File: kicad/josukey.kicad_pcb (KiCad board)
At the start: 2 copper layers, 150.9 x 94.8 mm, 44 parts

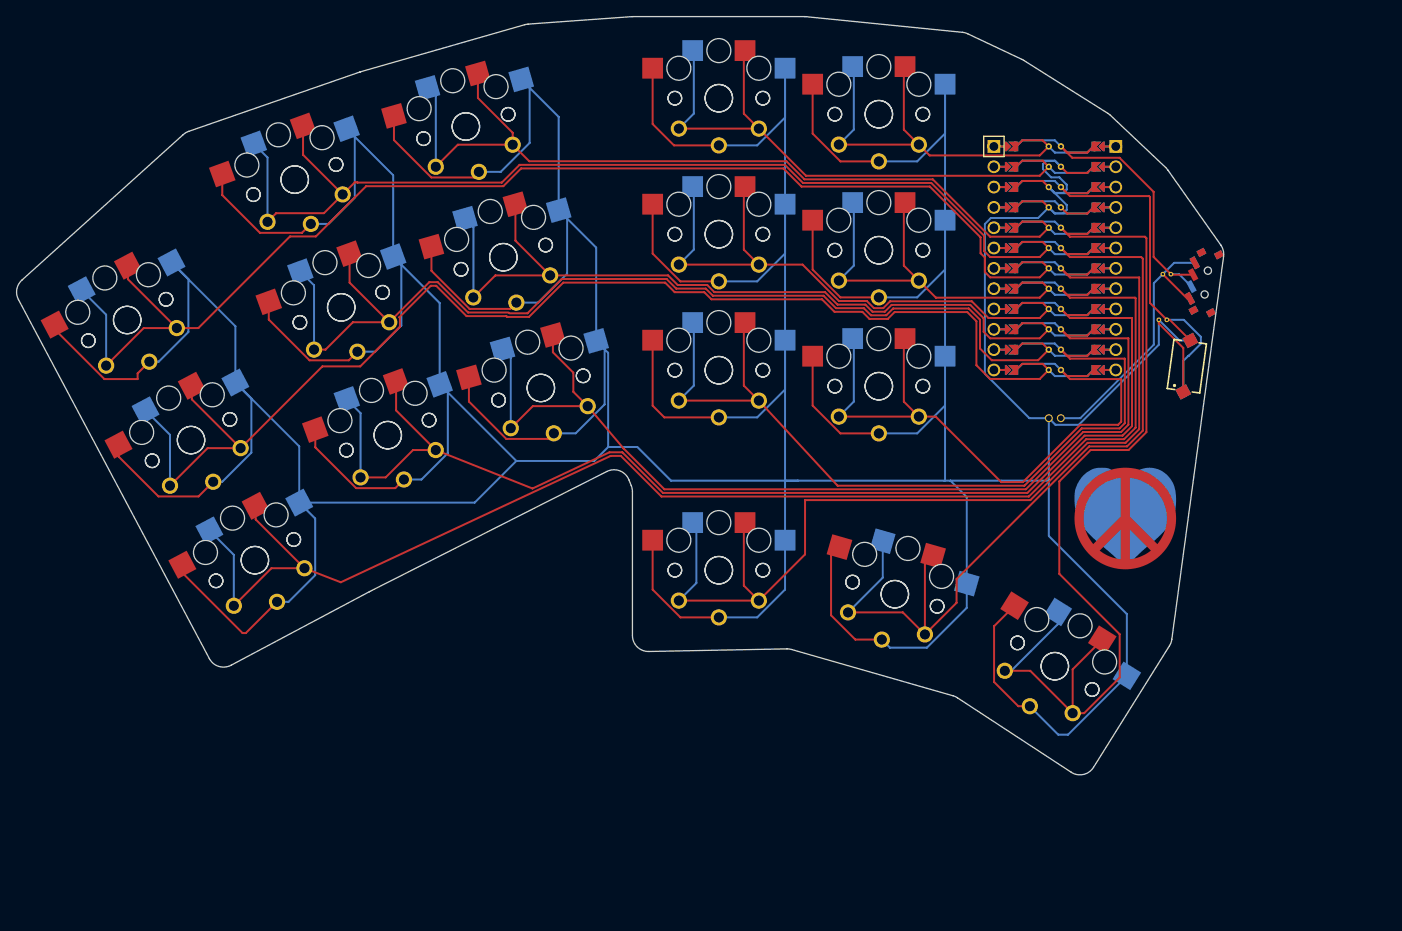
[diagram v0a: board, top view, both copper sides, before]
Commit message: add text and include images in ergogen config
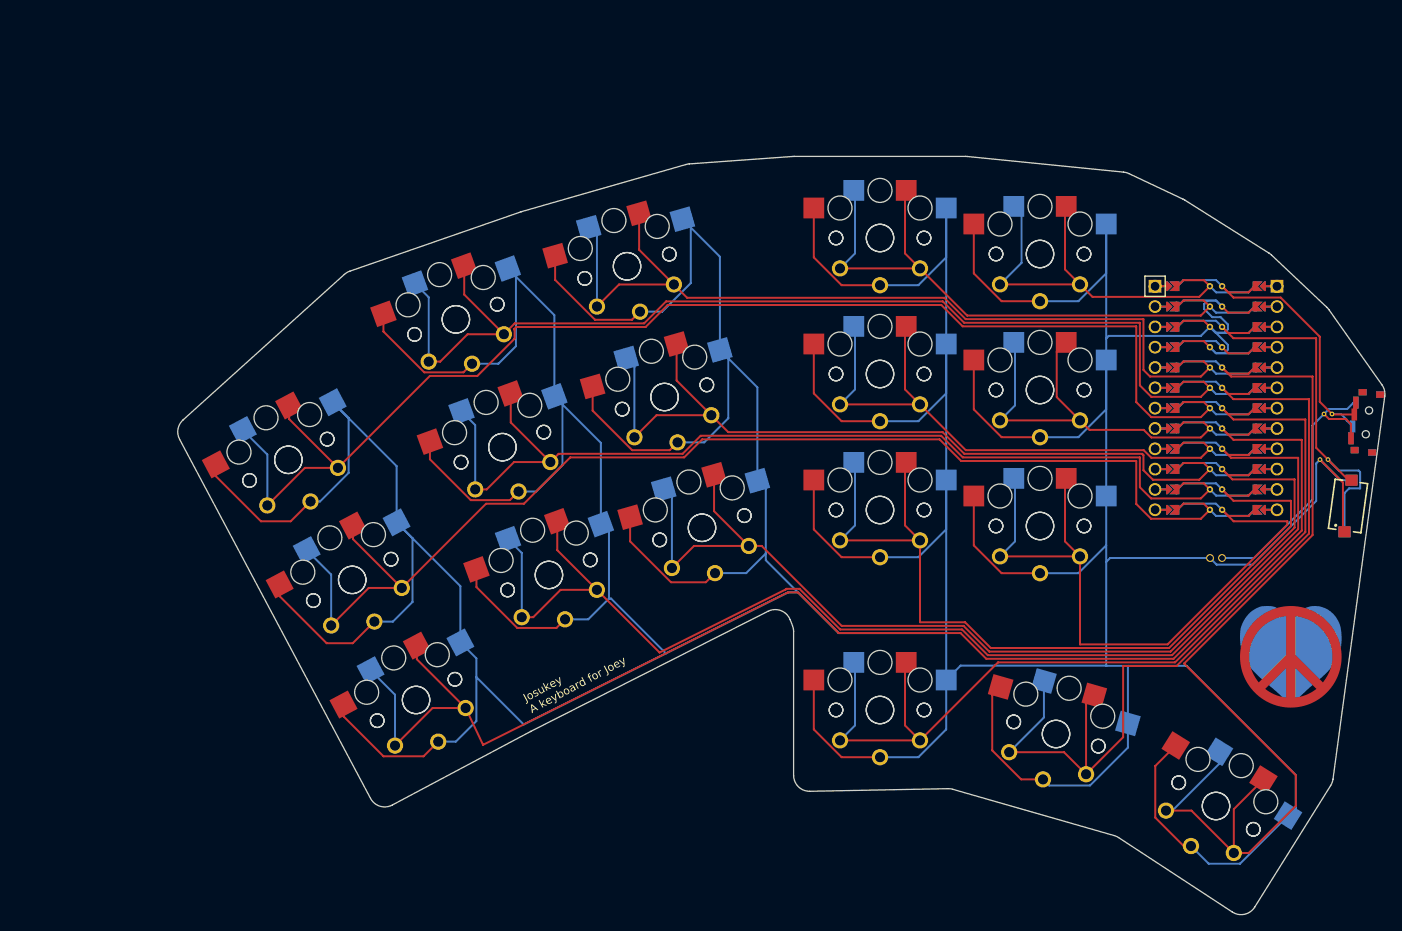
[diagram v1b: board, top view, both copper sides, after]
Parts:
- removed the REF** at (268.4, 138.6)
- removed the REF** at (267.9, 132.9)
- removed the REF** at (268.9, 132.9)
- removed the REF** at (267.4, 138.6)
- added REF**: VIA-0.6mm, VIA-0.6mm, F.Cu at (288.0, 150.4)
- added REF**: VIA-0.6mm, VIA-0.6mm, F.Cu at (289.0, 150.4)
- added REF**: VIA-0.6mm, VIA-0.6mm, F.Cu at (287.5, 156.1)
- added REF**: VIA-0.6mm, VIA-0.6mm, F.Cu at (288.5, 156.1)
- moved S12 26.7 mm to (232.5, 128.4)
- moved S30 26.7 mm to (232.5, 128.4)
- moved ? 26.7 mm to (291.0, 161.9)
- moved ? 26.7 mm to (274.5, 168.4)
- moved S14 26.7 mm to (252.5, 147.4)
- moved S17 26.7 mm to (254.5, 190.4)
- moved S21 26.7 mm to (158.5, 156.1)
- moved S22 26.7 mm to (191.1, 170.5)
- moved S25 26.7 mm to (210.2, 164.6)
- moved S3 26.7 mm to (158.5, 156.1)
- moved S32 26.7 mm to (252.5, 147.4)
- moved S35 26.7 mm to (254.5, 190.4)
- moved S4 26.7 mm to (191.1, 170.5)
- moved S7 26.7 mm to (210.2, 164.6)
- moved MCU1 26.7 mm to (274.5, 148.4)
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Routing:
- net GND: track 1060.6 -> 1025.1 mm
- net main_inner_bottom: track 76.3 -> 83.5 mm
- net main_pinky_home: track 154.8 -> 148.2 mm
- net main_index_bottom: track 101.3 -> 107.8 mm
- net thumb_inner_home: track 121.1 -> 115.2 mm
- net main_ring_home: track 127.2 -> 121.6 mm
- net main_pinky_bottom: track 171.2 -> 175.7 mm
- net main_pinky_top: track 157.4 -> 161.8 mm
- net main_ring_bottom: track 149.3 -> 153.6 mm
- net main_ring_top: track 128.1 -> 131.8 mm
- net thumb_outer_home: track 116.3 -> 120.0 mm
- net main_middle_top: track 104.0 -> 107.7 mm
- net pos: track 33.9 -> 35.9 mm
- net thumb_home_home: track 103.5 -> 105.5 mm
- net RST: track 44.8 -> 45.9 mm
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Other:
- board text added: "Josukey A keyboard for Joey"

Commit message: Restore former logo size. Update kicad with autorouted pcb
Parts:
- removed ?: , lib:bat
- removed ?: , 434121025816
- removed ?: , Button_Switch_SMD:SW_SPDT_PCM12
- removed REF** (x4): VIA-0.6mm, VIA-0.6mm
- removed S20, S21, S22, S23, S24, S25, S26, S27, S28, S29, S30, S31, S32, S33, S34, S35, S36: , PG1350
- added D1: Nexperia_CFP3_SOD-123W, Diode_SMD:Nexperia_CFP3_SOD-123W, F.Cu at (-7.60, 1.60)
- added D10: Nexperia_CFP3_SOD-123W, Diode_SMD:Nexperia_CFP3_SOD-123W, F.Cu at (46.4, -2.40)
- added D11: Nexperia_CFP3_SOD-123W, Diode_SMD:Nexperia_CFP3_SOD-123W, F.Cu at (46.4, -19.4)
- added D12: Nexperia_CFP3_SOD-123W, Diode_SMD:Nexperia_CFP3_SOD-123W, F.Cu at (46.4, -36.4)
- added D13: Nexperia_CFP3_SOD-123W, Diode_SMD:Nexperia_CFP3_SOD-123W, F.Cu at (64.4, -0.40)
- added D14: Nexperia_CFP3_SOD-123W, Diode_SMD:Nexperia_CFP3_SOD-123W, F.Cu at (64.4, -17.4)
- added D15: Nexperia_CFP3_SOD-123W, Diode_SMD:Nexperia_CFP3_SOD-123W, F.Cu at (64.4, -34.4)
- added D16: Nexperia_CFP3_SOD-123W, Diode_SMD:Nexperia_CFP3_SOD-123W, F.Cu at (37.4, 14.6)
- added D17: Nexperia_CFP3_SOD-123W, Diode_SMD:Nexperia_CFP3_SOD-123W, F.Cu at (57.3, 15.4)
- added D18: Nexperia_CFP3_SOD-123W, Diode_SMD:Nexperia_CFP3_SOD-123W, F.Cu at (75.9, 22.2)
- added D2: Nexperia_CFP3_SOD-123W, Diode_SMD:Nexperia_CFP3_SOD-123W, F.Cu at (-7.60, -15.4)
- added D3: Nexperia_CFP3_SOD-123W, Diode_SMD:Nexperia_CFP3_SOD-123W, F.Cu at (-7.60, -32.4)
- added D4: Nexperia_CFP3_SOD-123W, Diode_SMD:Nexperia_CFP3_SOD-123W, F.Cu at (10.4, -2.40)
- added D5: Nexperia_CFP3_SOD-123W, Diode_SMD:Nexperia_CFP3_SOD-123W, F.Cu at (10.4, -19.4)
- added D6: Nexperia_CFP3_SOD-123W, Diode_SMD:Nexperia_CFP3_SOD-123W, F.Cu at (10.4, -36.4)
- added D7: Nexperia_CFP3_SOD-123W, Diode_SMD:Nexperia_CFP3_SOD-123W, F.Cu at (28.4, -4.40)
- added D8: Nexperia_CFP3_SOD-123W, Diode_SMD:Nexperia_CFP3_SOD-123W, F.Cu at (28.4, -21.4)
- added D9: Nexperia_CFP3_SOD-123W, Diode_SMD:Nexperia_CFP3_SOD-123W, F.Cu at (28.4, -38.4)
- added LED1: , WS2812B, F.Cu at (0.00, 5.00)
- added LED10: , WS2812B, F.Cu at (54.0, 1.00)
- added LED11: , WS2812B, F.Cu at (54.0, -16.0)
- added LED12: , WS2812B, F.Cu at (54.0, -33.0)
- added LED13: , WS2812B, F.Cu at (72.0, 3.00)
- added LED14: , WS2812B, F.Cu at (72.0, -14.0)
- added LED15: , WS2812B, F.Cu at (72.0, -31.0)
- added LED16: , WS2812B, F.Cu at (45.0, 18.0)
- added LED17: , WS2812B, F.Cu at (63.5, 21.0)
- added LED18: , WS2812B, F.Cu at (80.1, 29.4)
- added LED2: , WS2812B, F.Cu at (0.00, -12.0)
- added LED3: , WS2812B, F.Cu at (0.00, -29.0)
- added LED4: , WS2812B, F.Cu at (18.0, 1.00)
- added LED5: , WS2812B, F.Cu at (18.0, -16.0)
- added LED6: , WS2812B, F.Cu at (18.0, -33.0)
- added LED7: , WS2812B, F.Cu at (36.0, -1.00)
- added LED8: , WS2812B, F.Cu at (36.0, -18.0)
- added LED9: , WS2812B, F.Cu at (36.0, -35.0)
- added T1: , Button_Switch_SMD:SW_SPDT_PCM12, F.Cu at (102.5, -5.00)
- added _1: , Connector_JST:JST_PH_S2B-PH-K_1x02_P2.00mm_Horizontal, F.Cu at (93.0, 0.00)
- S19: footprint PG1350 -> 434121025816
- moved S18 258.8 mm to (83.0, 25.4), turned to -36 degrees
- moved S17 257.4 mm to (65.0, 16.2), turned to -18 degrees
- moved S16 256.1 mm to (45.0, 13.0), turned to 0 degrees
- moved S1 255.2 mm to (0.00, 0.00), turned to 0 degrees
- moved S2 251.3 mm to (0.00, -17.0), turned to 0 degrees
- moved MCU1 250.7 mm to (94.0, -25.5)
- moved S3 247.6 mm to (0.00, -34.0), turned to 0 degrees
- moved S4 245.8 mm to (18.0, -4.00), turned to 0 degrees
- moved S13 245.5 mm to (72.0, -2.00), turned to 0 degrees
- moved S14 245.5 mm to (72.0, -19.0), turned to 0 degrees
- moved S15 245.5 mm to (72.0, -36.0), turned to 0 degrees
- moved S10 244.0 mm to (54.0, -4.00), turned to 0 degrees
- moved S11 244.0 mm to (54.0, -21.0), turned to 0 degrees
- moved S12 244.0 mm to (54.0, -38.0), turned to 0 degrees
- moved S7 243.9 mm to (36.0, -6.00), turned to 0 degrees
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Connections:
- MCU1 pad 10: main_middle_bottom -> P14
- MCU1 pad 11: main_index_bottom -> P16
- MCU1 pad 12: main_inner_bottom -> P10
- MCU1 pad 13: main_pinky_home -> P9
- MCU1 pad 14: main_ring_home -> P8
- MCU1 pad 15: main_middle_home -> P7
- MCU1 pad 16: main_index_home -> P6
- MCU1 pad 17: main_inner_home -> P5
- MCU1 pad 18: main_pinky_top -> P4
- MCU1 pad 19: main_ring_top -> P3
- MCU1 pad 20: main_middle_top -> P2
- MCU1 pad 23: main_index_top -> P0
- MCU1 pad 24: main_inner_top -> P1
- MCU1 pad 5: thumb_outer_home -> P21
- MCU1 pad 6: thumb_home_home -> P20
- MCU1 pad 7: thumb_inner_home -> P19
- MCU1 pad 8: main_pinky_bottom -> P18
- MCU1 pad 9: main_ring_bottom -> P15
- S1 pad 1: main_pinky_bottom -> P7
- S1 pad 2: GND -> main_pinky_bottom
- S10 pad 1: main_index_bottom -> P4
- S10 pad 2: GND -> main_index_bottom
- S11 pad 1: main_index_home -> P4
- S11 pad 2: GND -> main_index_home
- S12 pad 1: main_index_top -> P4
- S12 pad 2: GND -> main_index_top
- S13 pad 1: main_inner_bottom -> P3
- S13 pad 2: GND -> main_inner_bottom
- S14 pad 1: main_inner_home -> P3
- S14 pad 2: GND -> main_inner_home
- S15 pad 1: main_inner_top -> P3
- S15 pad 2: GND -> main_inner_top
- S16 pad 1: thumb_inner_home -> P5
- S16 pad 2: GND -> thumb_inner_home
- S17 pad 1: thumb_home_home -> P4
- S17 pad 2: GND -> thumb_home_home
- S18 pad 1: thumb_outer_home -> P3
- S18 pad 2: GND -> thumb_outer_home
- S19 pad 1: main_pinky_bottom -> RST
- S2 pad 1: main_pinky_home -> P7
- S2 pad 2: GND -> main_pinky_home
- S3 pad 1: main_pinky_top -> P7
- S3 pad 2: GND -> main_pinky_top
- S4 pad 1: main_ring_bottom -> P6
- S4 pad 2: GND -> main_ring_bottom
- S5 pad 1: main_ring_home -> P6
- S5 pad 2: GND -> main_ring_home
- S6 pad 1: main_ring_top -> P6
- S6 pad 2: GND -> main_ring_top
- S7 pad 1: main_middle_bottom -> P5
- S7 pad 2: GND -> main_middle_bottom
- S8 pad 1: main_middle_home -> P5
- S8 pad 2: GND -> main_middle_home
- S9 pad 1: main_middle_top -> P5
- S9 pad 2: GND -> main_middle_top
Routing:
- net VCC: track 0.00 -> 544.7 mm, vias 0 -> 15
- net GND: track 1025.1 -> 700.6 mm, vias 0 -> 9
- net P7: track 0.00 -> 199.8 mm, vias 0 -> 3
- net P4: track 0.00 -> 190.2 mm, vias 0 -> 5
- net P3: track 0.00 -> 174.0 mm, vias 0 -> 7
- net P5: track 0.00 -> 165.1 mm, vias 0 -> 6
- net P6: track 0.00 -> 151.6 mm, vias 0 -> 5
- net main_pinky_bottom: track 175.7 -> 24.7 mm, vias 0 -> 1
- net P2: track 0.00 -> 142.5 mm, vias 0 -> 1
- net main_pinky_top: track 161.8 -> 21.9 mm
- net P0: track 0.00 -> 132.2 mm, vias 0 -> 3
- net main_ring_bottom: track 153.6 -> 23.2 mm, vias 0 -> 1
- net main_pinky_home: track 148.2 -> 22.8 mm, vias 0 -> 1
- net P1: track 0.00 -> 117.8 mm, vias 0 -> 1
- net P8: track 0.00 -> 105.6 mm, vias 0 -> 2
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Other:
- board size 150.9 x 94.8 mm -> 115.2 x 89.6 mm
